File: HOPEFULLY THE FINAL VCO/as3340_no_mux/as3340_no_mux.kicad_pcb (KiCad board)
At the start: 2 copper layers, 55.8 x 128.5 mm, 85 parts, among them J1 Sync INput, J11 Conn_02x05_Odd_Even, J12 TRI OUt, J13 SIN OUT, J14 SAW OUt, J15 SQR OUT, J2 CV1, J4 LinearFmINput, J5 PWM INput, SW1 SW_SPDT, U1 LM13700, U2 AS3340, U4 LM324

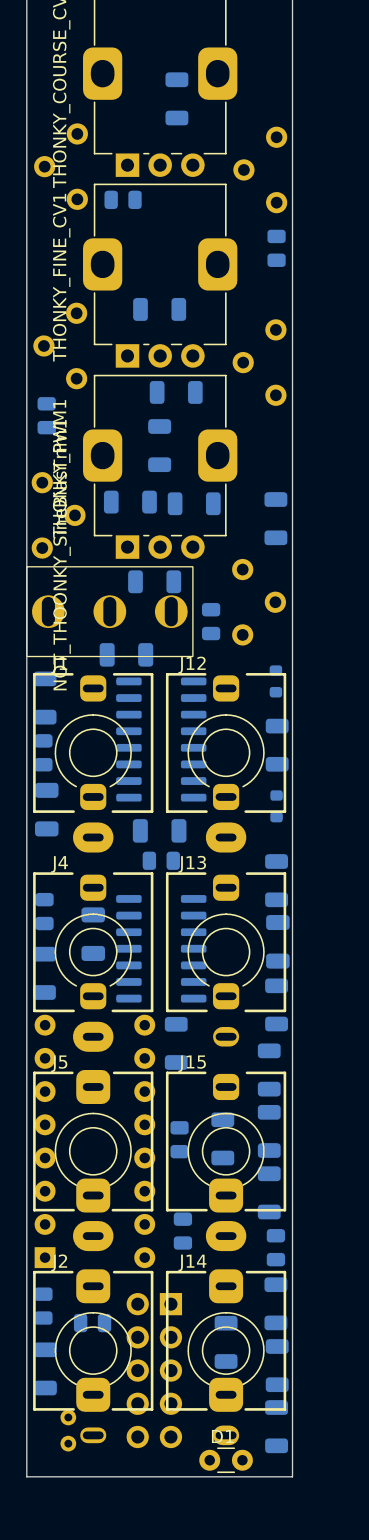
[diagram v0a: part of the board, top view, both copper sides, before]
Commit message: hhgreg
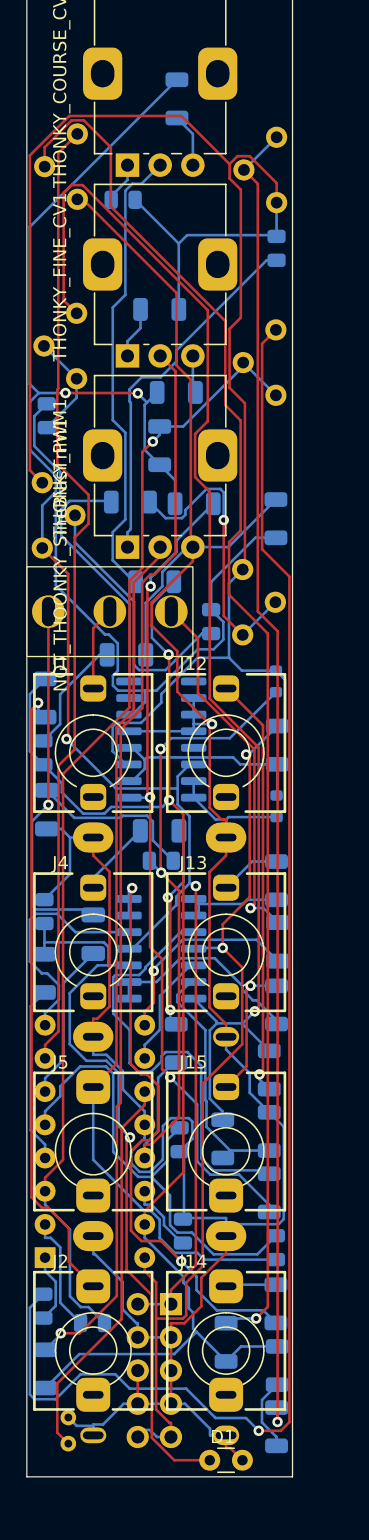
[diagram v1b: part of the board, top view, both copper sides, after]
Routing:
- net GND: track 0.00 -> 236.3 mm, vias 0 -> 1
- net +15V: track 0.00 -> 205.1 mm, vias 0 -> 2
- net -15V: track 0.00 -> 139.4 mm, vias 0 -> 4
- net Net-(NOT_THINKY_TEMKO1-Pad1): track 0.00 -> 115.8 mm, vias 0 -> 1
- net Net-(NOT_THONKY_HF_TRACK1-Pad2): track 0.00 -> 106.3 mm, vias 0 -> 1
- net Net-(U2-VFCI): track 0.00 -> 102.3 mm, vias 0 -> 2
- net Net-(NOT+THINKY_CV1-Pad1): track 0.00 -> 101.5 mm, vias 0 -> 1
- net Net-(NOT_THONKY_SineShapeTrim1-Pad1): track 0.00 -> 97.9 mm, vias 0 -> 1
- net Net-(U2-VEE): track 0.00 -> 86.4 mm, vias 0 -> 1
- net Net-(R19-Pad1): track 0.00 -> 81.6 mm, vias 0 -> 1
- net Net-(U2-VHFT): track 0.00 -> 73.7 mm
- net Net-(J5-PadR): track 0.00 -> 66.9 mm
- net Net-(R3-Pad1): track 0.00 -> 63.0 mm, vias 0 -> 3
- net Net-(D1-A): track 0.00 -> 57.1 mm, vias 0 -> 1
- net Net-(U2-VLFI): track 0.00 -> 53.6 mm, vias 0 -> 2
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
